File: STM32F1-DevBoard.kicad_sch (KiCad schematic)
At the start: 26 parts, among them SW1 SW_Push, SW2 SW_Push, U1 STM32F103C8T6, U2 AMS1117-3.3

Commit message: Add files via upload
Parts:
- U1: JLCPCB Rotation Offset (none) -> -90
- U2: JLCPCB Rotation Offset (none) -> -180
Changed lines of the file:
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@@
+      (effects (font (size 1.27 1.27)) hide)
+    )
+    (property "JLCPCB Rotation Offset" "-90" (at 67.31 110.49 0)
       (effects (font (size 1.27 1.27)) hide)
     )
@@
       (effects (font (size 1.27 1.27)) hide)
     )
+    (property "JLCPCB Rotation Offset" "-180" (at 116.84 35.56 0)
+      (effects (font (size 1.27 1.27)) hide)
+    )

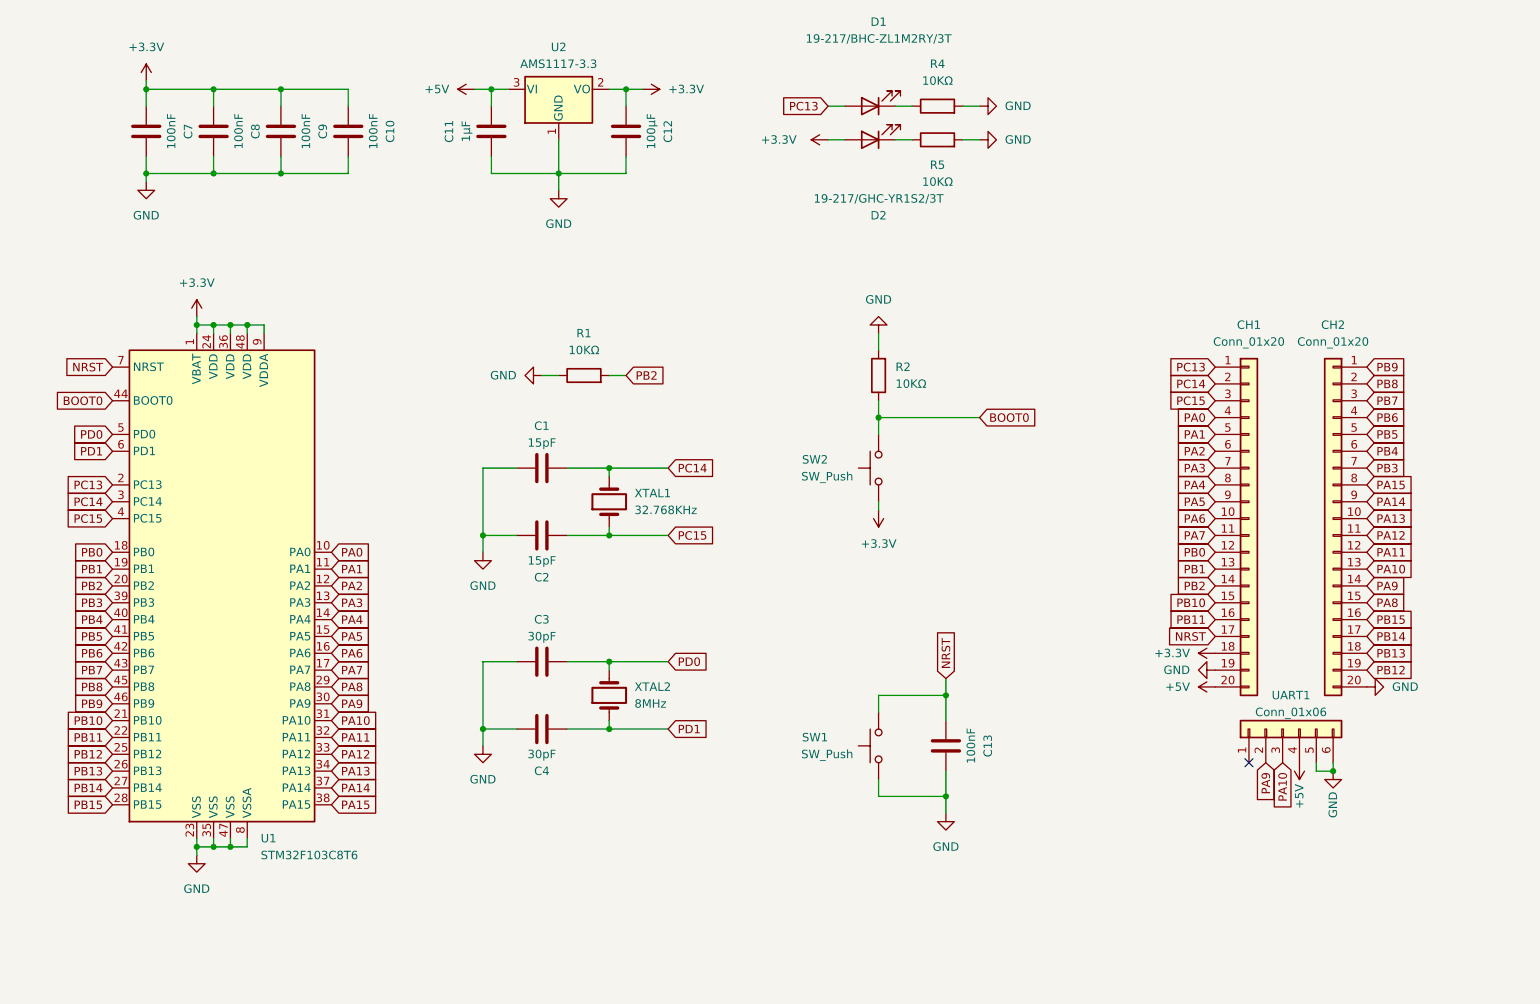
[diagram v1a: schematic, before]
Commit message: Add files via upload
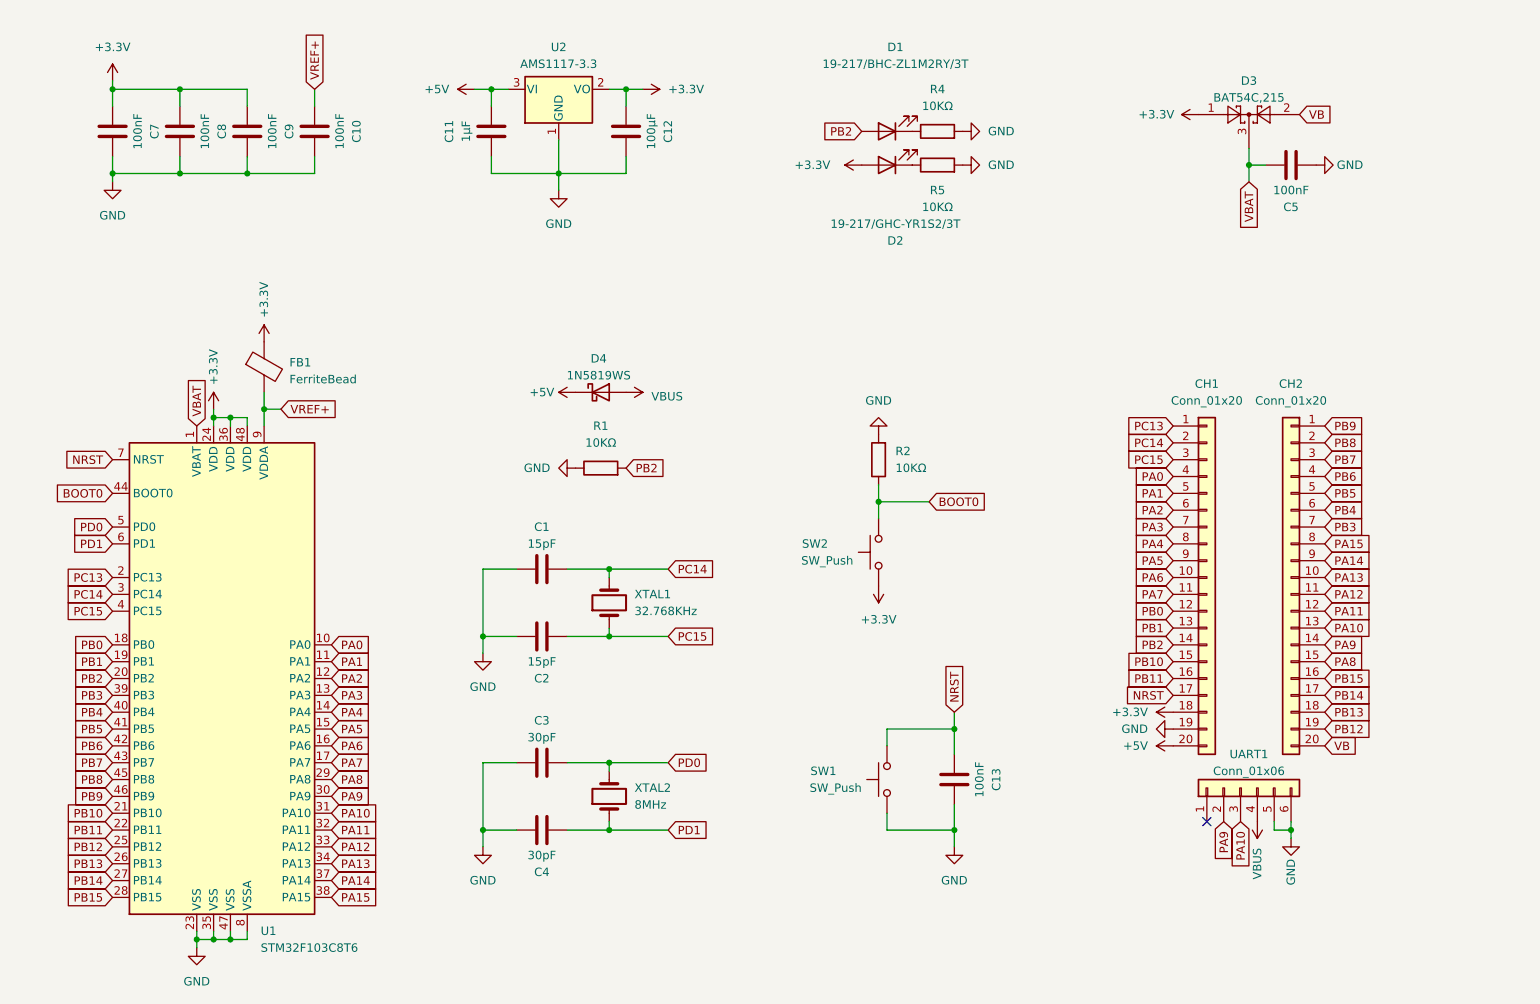
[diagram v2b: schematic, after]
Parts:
- added C5: 100nF, Capacitor_SMD:C_0402_1005Metric, symbol Device:C
- added D3: BAT54C,215, Package_TO_SOT_SMD:SOT-23, symbol Diode:BAT54C
- added D4: 1N5819WS, Diode_SMD:D_SOD-323, symbol Diode:1N5819WS
- added FB1: FerriteBead, Inductor_SMD:L_0603_1608Metric, symbol Device:FerriteBead
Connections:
- net +3.3V: now also D3.1, FB1.1; no longer C10.1, U1.1 (VBAT), U1.9 (VDDA)
- net +5V: now also D4.1 (K); no longer UART1.4 (Pin_4)
- net GND: now also C5.1; no longer CH2.20 (Pin_20)
- net PB2: now also D1.2 (A)
- net PC13: no longer D1.2 (A)
- new net VB: CH2.20 (Pin_20), D3.2
- new net VBAT: C5.2, D3.3, U1.1 (VBAT)
- new net VBUS: D4.2 (A), UART1.4 (Pin_4)
- new net VREF+: C10.1, FB1.2, U1.9 (VDDA)
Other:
- moved on the sheet: C1, C10, C13, C2, C3, C4, C7, C8, C9, CH1, CH2, D1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

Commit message: Add files via upload
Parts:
- XTAL1, XTAL2: JLCPCB Rotation Offset (none) -> -180
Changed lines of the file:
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@@
+      (effects (font (size 1.27 1.27)) hide)
+    )
+    (property "JLCPCB Rotation Offset" "-180" (at 124.46 113.03 90)
       (effects (font (size 1.27 1.27)) hide)
     )
@@
       (effects (font (size 1.27 1.27)) hide)
     )
+    (property "JLCPCB Rotation Offset" "-180" (at 124.46 142.24 90)
+      (effects (font (size 1.27 1.27)) hide)
+    )

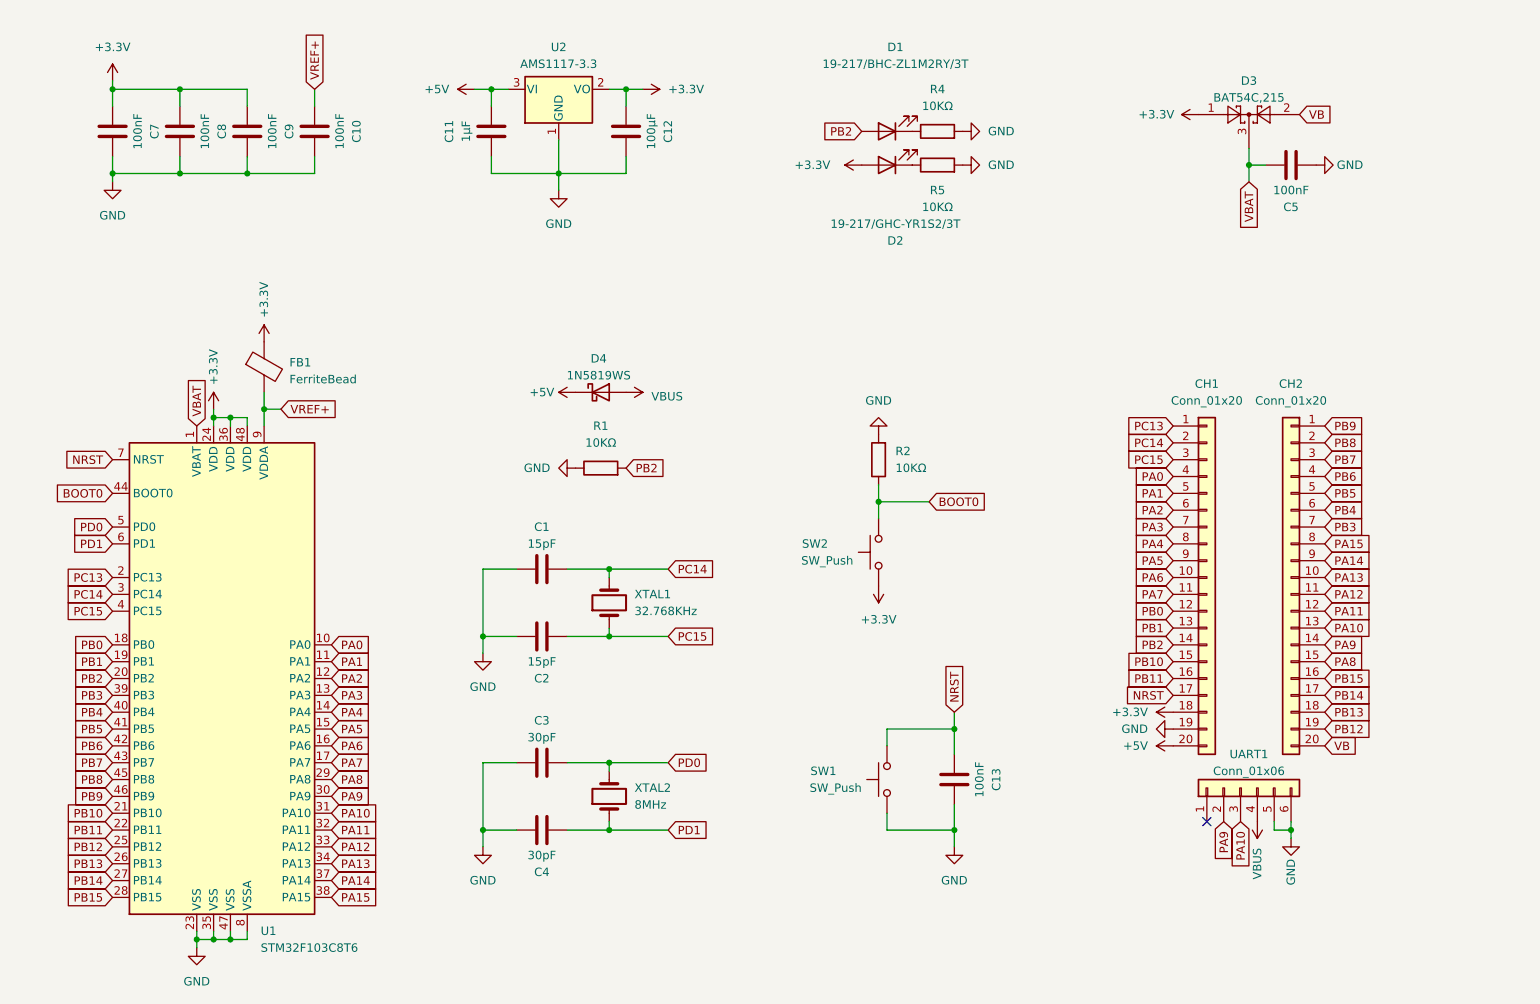
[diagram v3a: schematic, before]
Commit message: Add files via upload
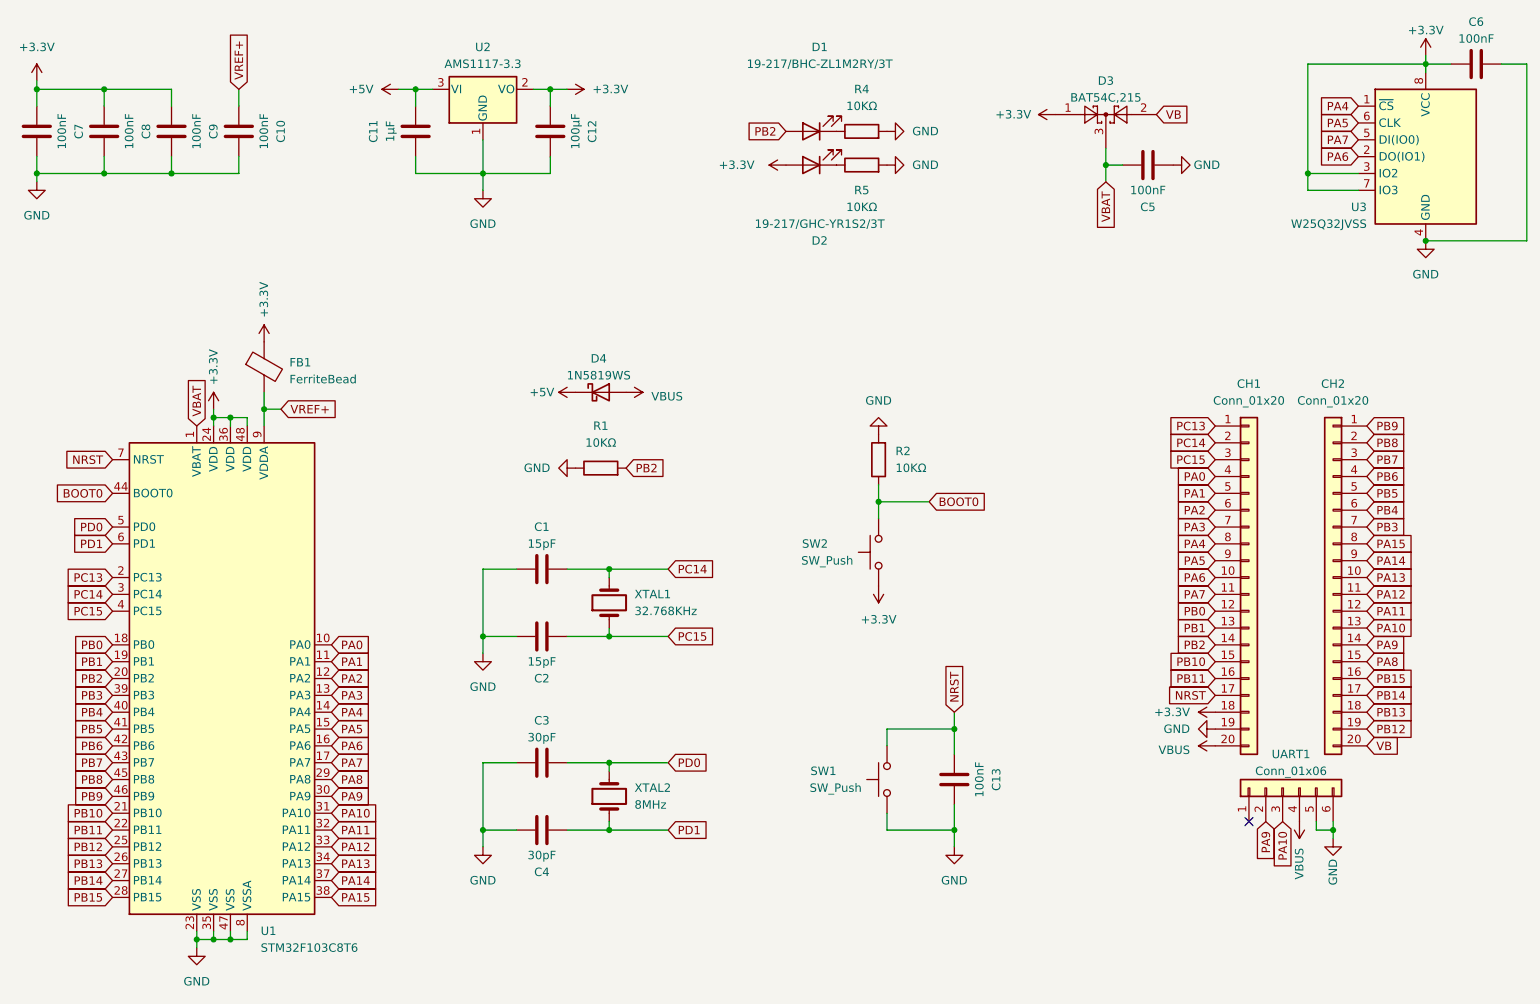
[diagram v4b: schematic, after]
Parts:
- added C6: 100nF, Capacitor_SMD:C_0603_1608Metric, symbol Device:C
- added U3: W25Q32JVSS, Package_SO:SOIC-8_5.23x5.23mm_P1.27mm, symbol Memory_Flash:W25Q32JVSS
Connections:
- net +3.3V: now also C6.1, U3.3 (IO2), U3.7 (IO3), U3.8 (VCC)
- net +5V: no longer CH1.20 (Pin_20)
- net GND: now also C6.2, U3.4 (GND)
- net PA4: now also U3.1 (~{CS})
- net PA5: now also U3.6 (CLK)
- net PA6: now also U3.2 (DO(IO1))
- net PA7: now also U3.5 (DI(IO0))
- net VBUS: now also CH1.20 (Pin_20)
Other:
- moved on the sheet: C10, C11, C12, C5, C7, C8, C9, CH1, CH2, D1, D2, D3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
